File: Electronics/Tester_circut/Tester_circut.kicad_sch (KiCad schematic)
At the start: 14 parts, among them Q1 BC547

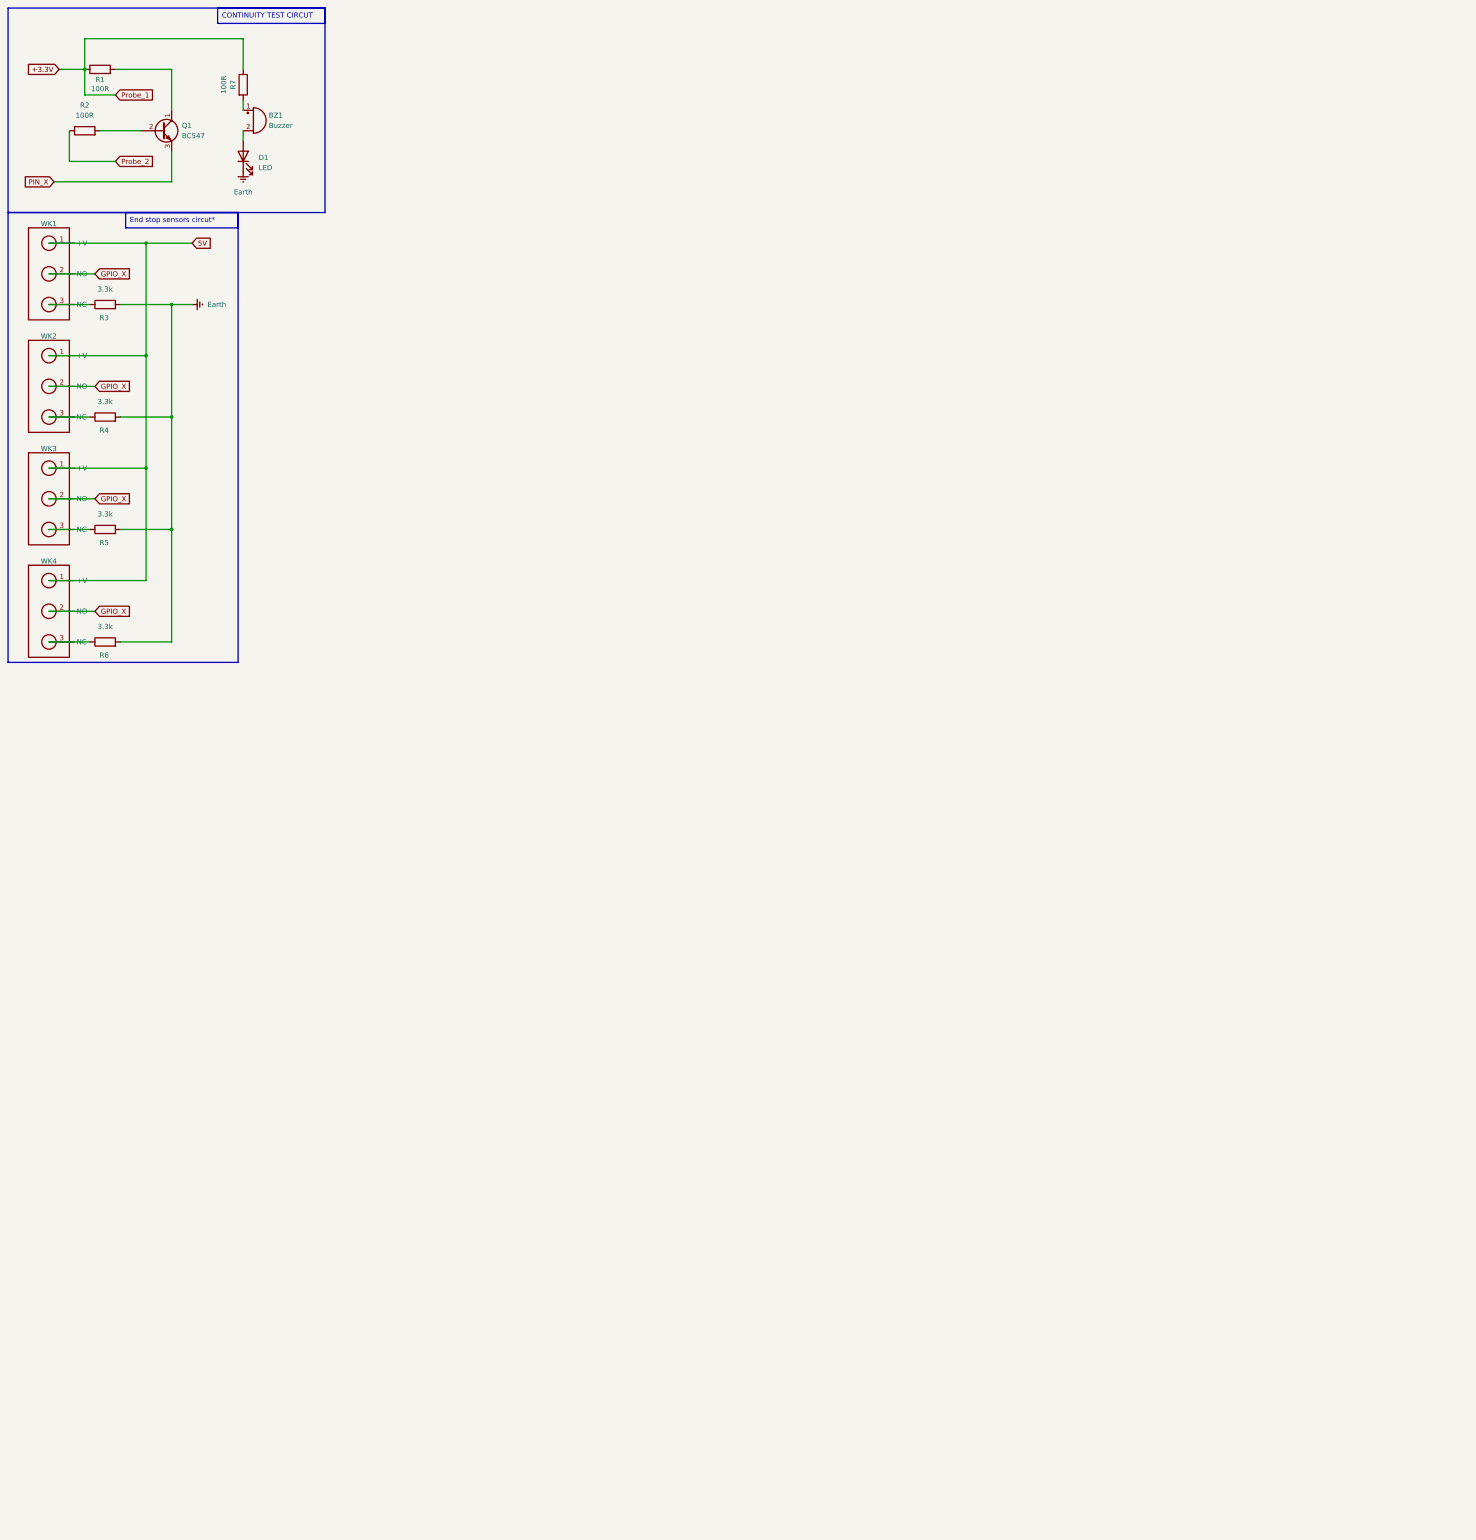
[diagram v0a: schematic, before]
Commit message: PCB and schematics update
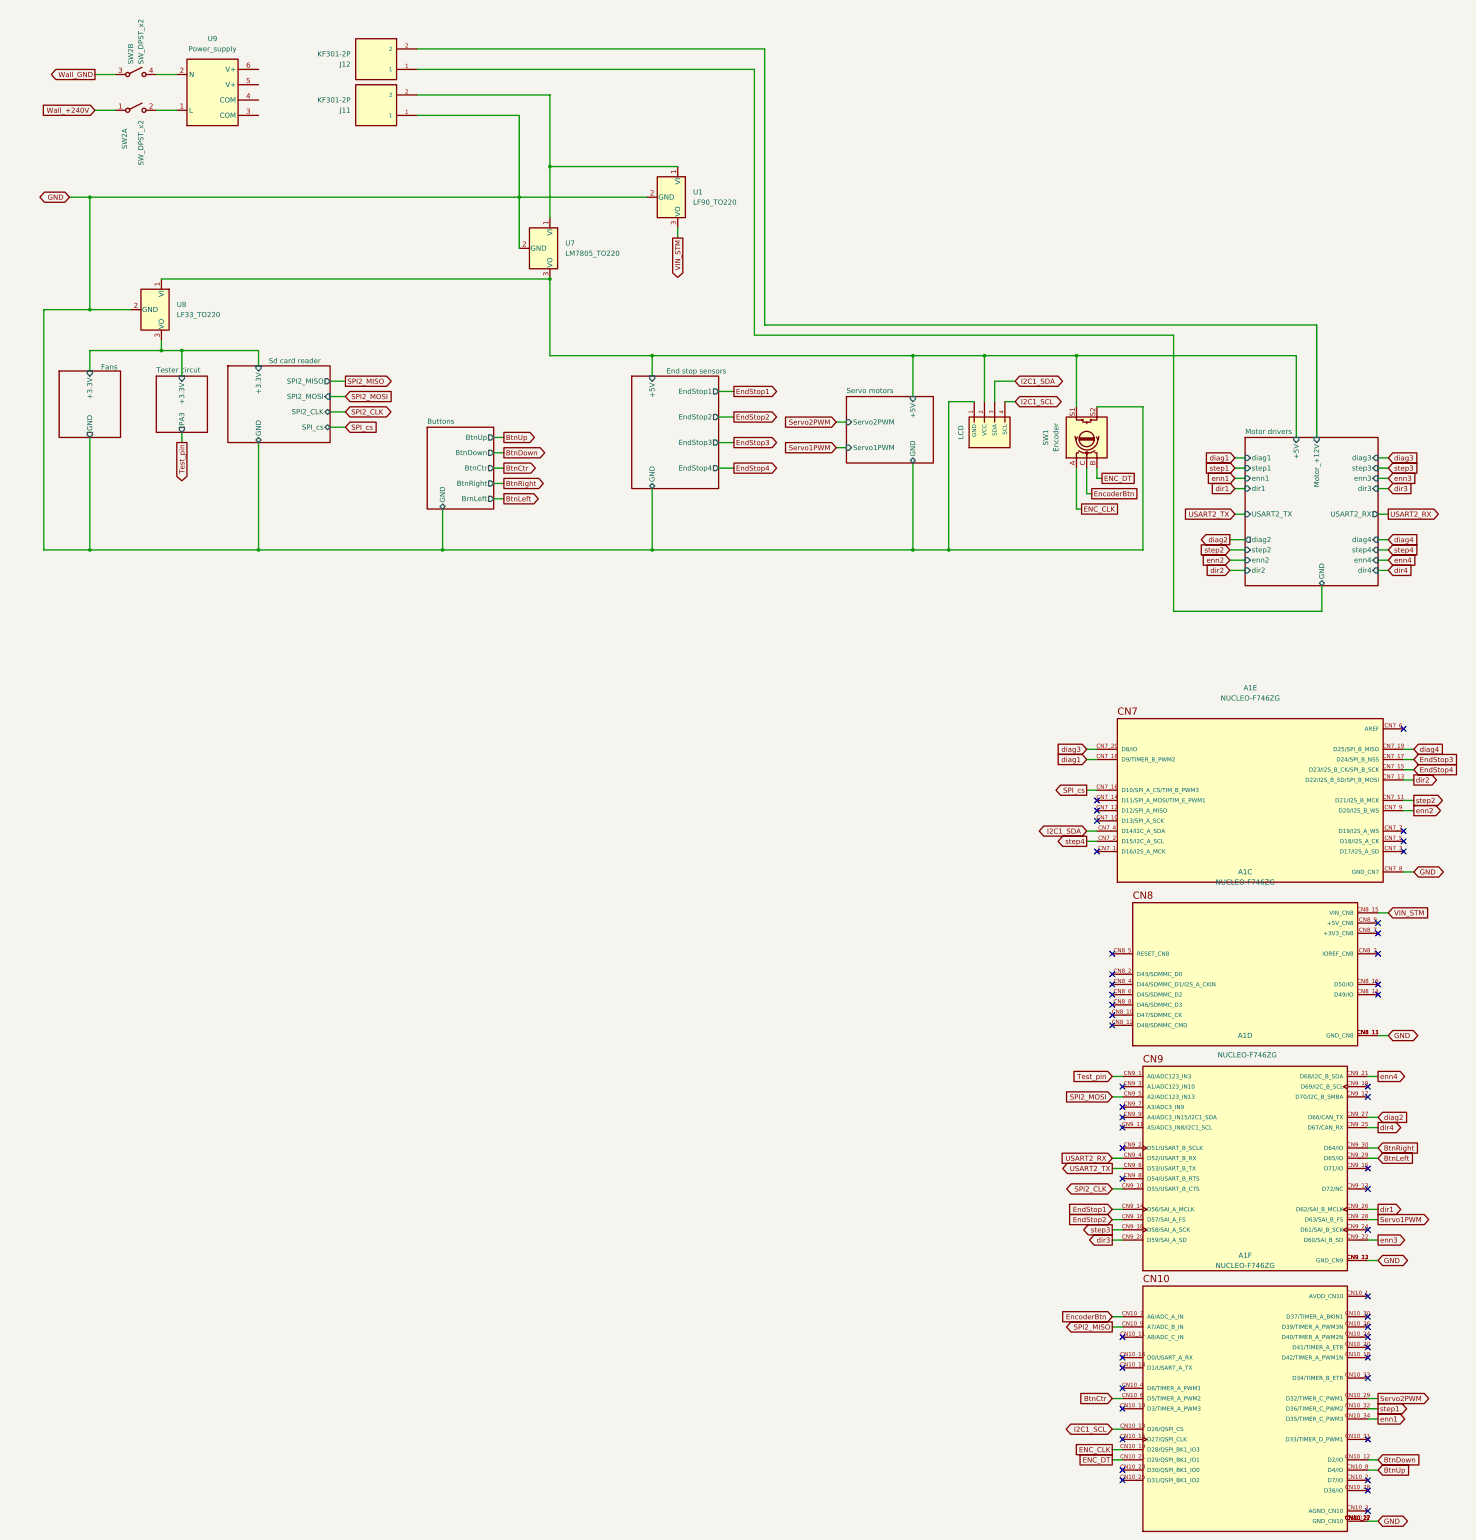
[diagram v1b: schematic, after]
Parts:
- removed BZ1: Buzzer, symbol Device:Buzzer
- removed D1: LED, symbol Device:LED
- removed Q1: BC547, Package_TO_SOT_THT:TO-92_Inline, symbol Transistor_BJT:BC547
- removed R1, R2, R7: 100R, symbol Device:R
- removed R3, R4, R5, R6: 3.3k, symbol Device:R
- removed WK1, WK2, WK3, WK4: ~, symbol Sensor:End_stop_mechanical_sensor
- added A1: NUCLEO-F746ZG, NUCLEO-F746ZG:MODULE_NUCLEO-F746ZG, symbol NUCLEO-F746ZG:NUCLEO-F746ZG
- added J11, J12: KF301-2P, KF301-2P:HANDSON_KF301-2P, symbol KF301-2P:KF301-2P
- added SW1: Encoder, Library:encoder, symbol Device:RotaryEncoder_Switch
- added SW2: SW_DPST_x2, symbol Switch:SW_DPST_x2
- added U1: LF90_TO220, Package_TO_SOT_THT:TO-220-3_Vertical, symbol Regulator_Linear:LF90_TO220
- added U4: LCD, Library:LCD, symbol TMC2209_SILENTSTEPSTICK:LCD
- added U7: LM7805_TO220, Package_TO_SOT_THT:TO-220-3_Vertical, symbol Regulator_Linear:LM7805_TO220
- added U8: LF33_TO220, Package_TO_SOT_THT:TO-220-3_Vertical, symbol Regulator_Linear:LF33_TO220
- added U9: Power_supply, Library:POWER_SUPPLY, symbol Converter_ACDC:U
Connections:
- new net: SW2.4 (B), U9.2 (N)
- new net: J11.2, U1.1 (VI), U7.1 (VI)
- new net: SW2.2 (B), U9.1 (L)
- new net BtnCtr: A1.CN10_6 (D5/TIMER_A_PWM2)
- new net BtnDown: A1.CN10_12 (D2/IO)
- new net BtnLeft: A1.CN9_29 (D65/IO)
- new net BtnRight: A1.CN9_30 (D64/IO)
- new net BtnUp: A1.CN10_8 (D4/IO)
- new net ENC_CLK: A1.CN10_19 (D28/QSPI_BK1_IO3), SW1.A
- new net ENC_DT: A1.CN10_21 (D29/QSPI_BK1_IO1), SW1.B
- new net EncoderBtn: A1.CN10_7 (A6/ADC_A_IN), SW1.C
- new net End stop sensors/+5V: SW1.S1, U4.2 (VCC), U7.3 (VO), U8.1 (VI)
- new net EndStop1: A1.CN9_14 (D56/SAI_A_MCLK)
- new net EndStop2: A1.CN9_16 (D57/SAI_A_FS)
- new net EndStop3: A1.CN7_17 (D24/SPI_B_NSS)
- new net EndStop4: A1.CN7_15 (D23/I2S_B_CK/SPI_B_SCK)
- new net Fans/+3.3V: U8.3 (VO)
- new net GND: A1.CN10_17 (GND_CN10), A1.CN10_22 (GND_CN10), A1.CN10_27 (GND_CN10), A1.CN10_5 (GND_CN10), A1.CN7_8 (GND_CN7), A1.CN8_11 (GND_CN8), A1.CN8_13 (GND_CN8), A1.CN9_12 (GND_CN9), A1.CN9_23 (GND_CN9), J11.1, SW1.S2, U1.2 (GND), U4.1 (GND), U7.2 (GND), U8.2 (GND)
- new net I2C1_SCL: A1.CN10_13 (D26/QSPI_CS), U4.4 (SCL)
- new net I2C1_SDA: A1.CN7_4 (D14/I2C_A_SDA), U4.3 (SDA)
- new net Motor drivers/GND: J12.1
- new net Motor drivers/Motor_+12V: J12.2
- new net SPI2_CLK: A1.CN9_10 (D55/USART_B_CTS)
- new net SPI2_MISO: A1.CN10_9 (A7/ADC_B_IN)
- new net SPI2_MOSI: A1.CN9_5 (A2/ADC123_IN13)
- new net SPI_cs: A1.CN7_16 (D10/SPI_A_CS/TIM_B_PWM3)
- new net Servo1PWM: A1.CN9_28 (D63/SAI_B_FS)
- new net Servo2PWM: A1.CN10_29 (D32/TIMER_C_PWM1)
- new net Test_pin: A1.CN9_1 (A0/ADC123_IN3)
- new net USART2_RX: A1.CN9_4 (D52/USART_B_RX)
- new net USART2_TX: A1.CN9_6 (D53/USART_B_TX)
- new net VIN_STM: A1.CN8_15 (VIN_CN8), U1.3 (VO)
- new net Wall_+240V: SW2.1 (A)
- new net Wall_GND: SW2.3 (A)
- new net diag1: A1.CN7_18 (D9/TIMER_B_PWM2)
- new net diag2: A1.CN9_27 (D66/CAN_TX)
- new net diag3: A1.CN7_20 (D8/IO)
- new net diag4: A1.CN7_19 (D25/SPI_B_MISO)
- new net dir1: A1.CN9_26 (D62/SAI_B_MCLK)
- new net dir2: A1.CN7_13 (D22/I2S_B_SD/SPI_B_MOSI)
- new net dir3: A1.CN9_20 (D59/SAI_A_SD)
- new net dir4: A1.CN9_25 (D67/CAN_RX)
- new net enn1: A1.CN10_34 (D35/TIMER_C_PWM3)
- new net enn2: A1.CN7_9 (D20/I2S_B_WS)
- new net enn3: A1.CN9_22 (D60/SAI_B_SD)
- new net enn4: A1.CN9_21 (D68/I2C_B_SDA)
- new net step1: A1.CN10_32 (D36/TIMER_C_PWM2)
- new net step2: A1.CN7_11 (D21/I2S_B_MCK)
- new net step3: A1.CN9_18 (D58/SAI_A_SCK)
- new net step4: A1.CN7_2 (D15/I2C_A_SCL)
- no-connect marks 0 -> 50
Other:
- added sheet Buttons (buttons.kicad_sch)
- added sheet End stop sensors (endstop.kicad_sch)
- added sheet Fans (Fans.kicad_sch)
- added sheet Motor drivers (Motor_drivers.kicad_sch)
- added sheet Sd card reader (sdreader.kicad_sch)
- added sheet Servo motors (servo.kicad_sch)
- added sheet Tester circut (untitled.kicad_sch)
- title: (none) -> Flying probe tester - PCB shield for STM32F746ZG
